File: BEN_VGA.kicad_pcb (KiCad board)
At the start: 4 copper layers, 135.3 x 95.9 mm, 57 parts, among them J1 VGA, J2 GND 5v, U1 74LS161, U10 74LS00, U11 74LS161, U12 74LS161, U13 74LS161, U14 74LS04, U15 74LS04, U16 74LS30, U17 74LS30, U18 74LS30, U19 74LS30, U2 74LS161, U20 74LS00, U22 28C256, U23 74LS00, U3 74LS161, U4 74LS04, U5 74LS04, U6 74LS30, U7 74LS30, U8 74LS30, U9 74LS30, X1 CXO_DIP14

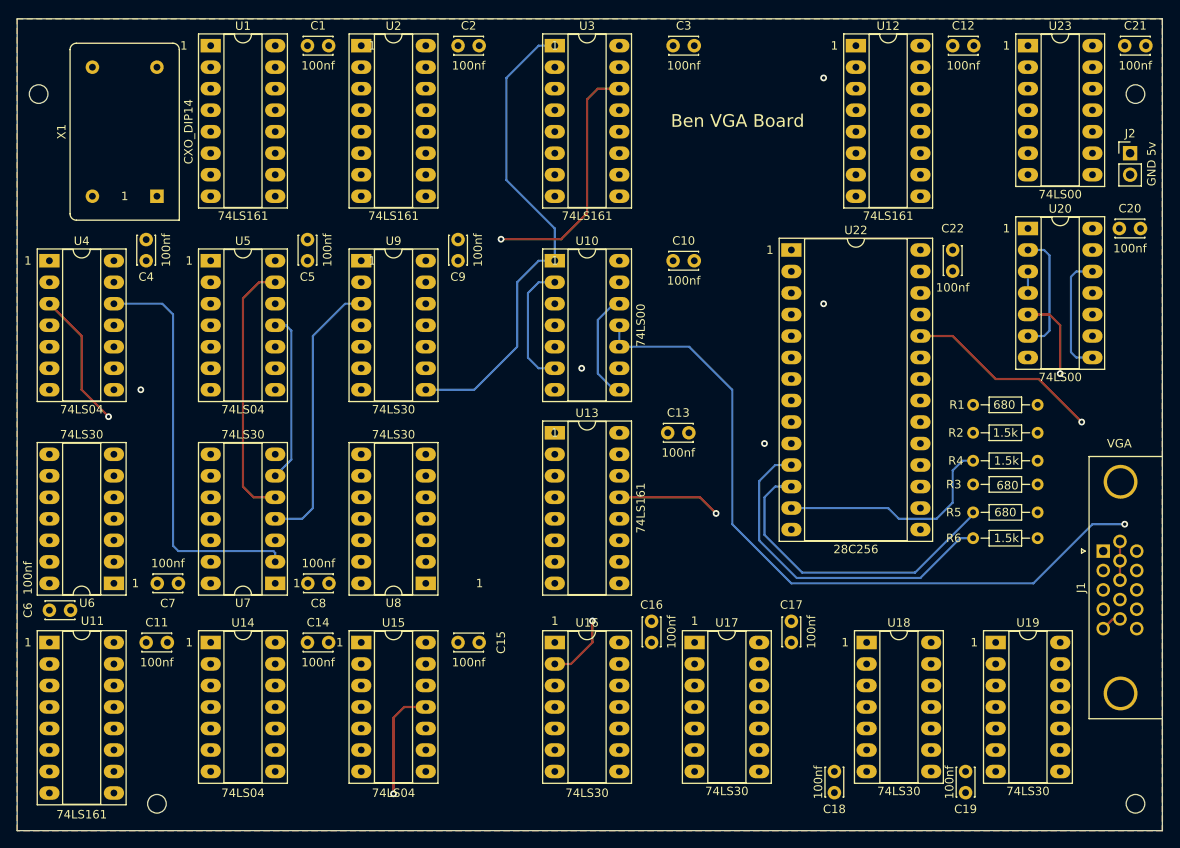
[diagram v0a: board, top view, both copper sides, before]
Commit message: shrink the board
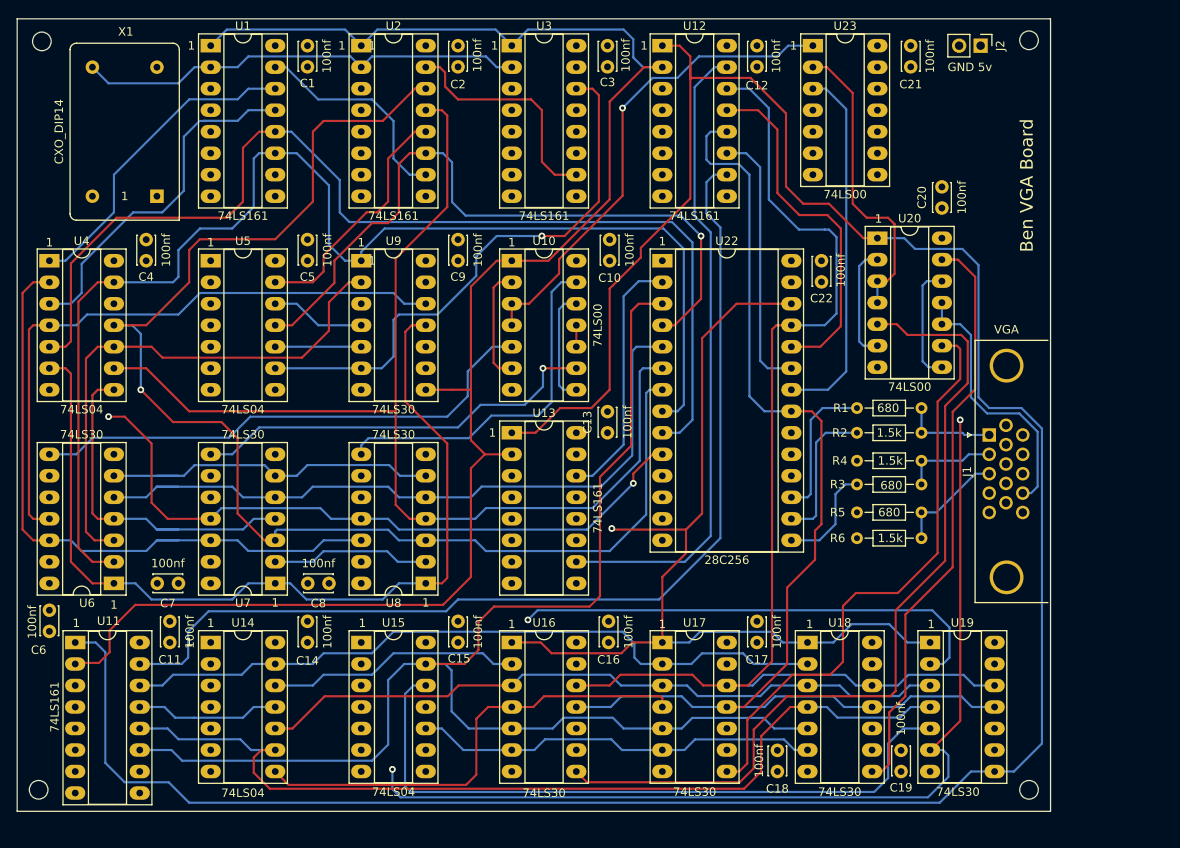
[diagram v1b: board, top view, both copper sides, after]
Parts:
- moved U23 25.4 mm to (188.0, 69.8)
- moved C21 25.3 mm to (199.5, 69.8), turned to 270 degrees
- moved C12 23.1 mm to (181.4, 69.8), turned to 270 degrees
- moved U12 22.9 mm to (170.2, 69.8)
- moved J2 21.7 mm to (207.8, 69.8), turned to 270 degrees
- moved C20 21.1 mm to (203.2, 89.0), turned to 90 degrees
- moved J1 19.2 mm to (208.8, 115.8)
- moved U20 17.8 mm to (195.6, 92.6)
- moved C22 15.5 mm to (189.0, 95.2)
- moved U22 15.3 mm to (170.2, 95.2)
- moved H3 14.1 mm to (213.5, 69.2)
- moved H2 14.1 mm to (96.5, 157.7)
- moved R1 13.7 mm to (193.2, 112.6)
- moved R2 13.7 mm to (193.2, 115.6)
- moved R3 13.7 mm to (193.2, 121.7)
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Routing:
- net /HSync/264: track 246.3 -> 197.1 mm
- net Net-(U11-Pad1): track 345.4 -> 305.6 mm
- net /HSync/HBLANK: track 77.0 -> 57.8 mm
- net /VSync/Q3: track 180.9 -> 161.7 mm
- net Net-(U11-Pad15): track 140.5 -> 122.0 mm
- net VSYNC: track 48.4 -> 32.0 mm
- net /HSync/Q4: track 173.1 -> 158.3 mm
- net /VSync/Q2: track 124.7 -> 110.0 mm
- net /HSync/Q6: track 158.1 -> 143.6 mm
- net /HSync/Q5: track 146.5 -> 132.4 mm
- net Net-(J1-Pad1): track 24.3 -> 10.9 mm
- net /HSync/Q2: track 141.6 -> 128.4 mm
- net /VSync/Q5: track 204.4 -> 191.5 mm
- net /HSync/Q1: track 153.9 -> 141.3 mm
- net /HSync/Q3: track 163.2 -> 151.7 mm
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- added copper zone on In2.Cu, net +5V
- added copper zone on In1.Cu, net GND
- removed copper zone on B.Cu, net +5V
- removed copper zone on F.Cu, net GND
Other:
- board size 135.3 x 95.9 mm -> 122 x 93.6 mm
